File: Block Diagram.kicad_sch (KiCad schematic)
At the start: 0 parts

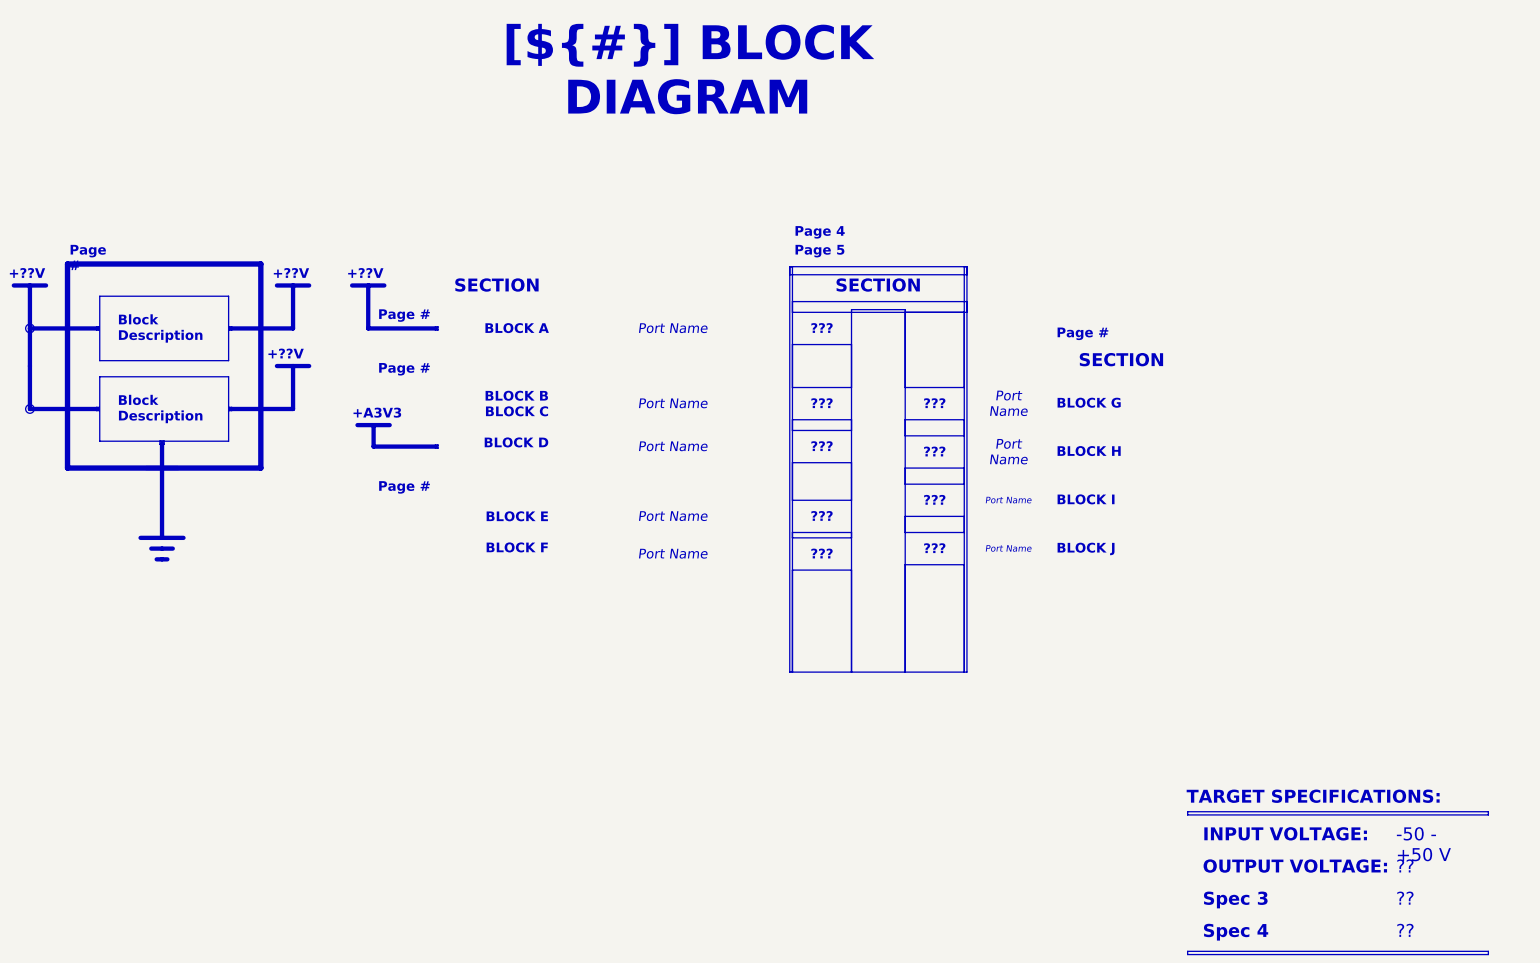
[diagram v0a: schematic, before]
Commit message: fix: template changes
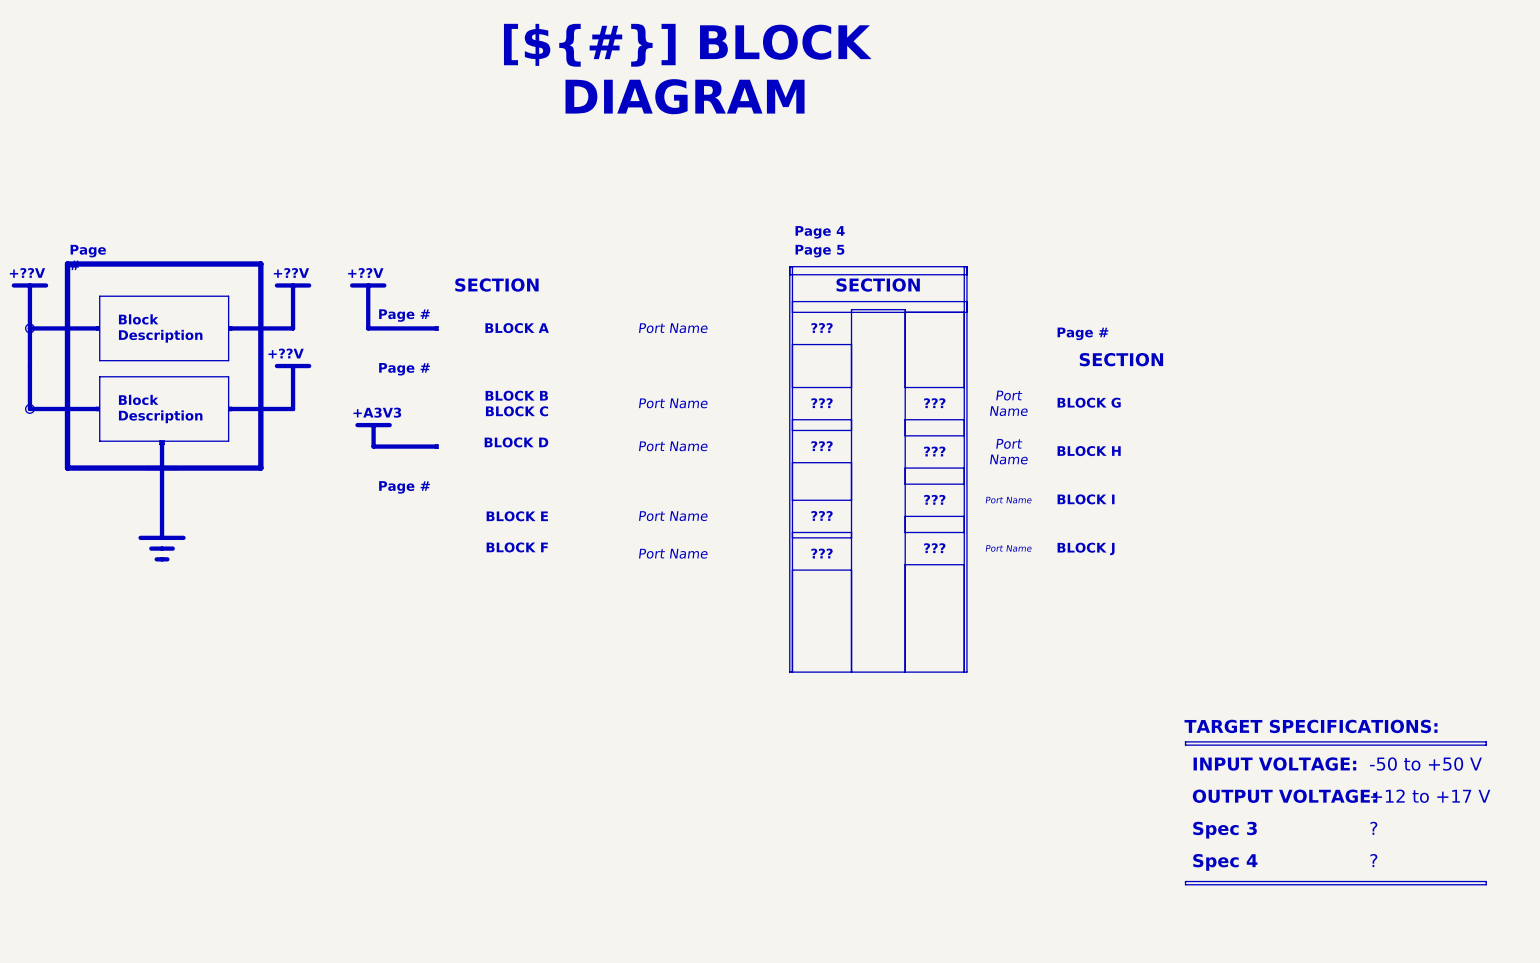
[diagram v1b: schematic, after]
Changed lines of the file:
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@@
 	)
 	(rectangle
-		(start 328.422 234.95)
-		(end 399.542 235.712)
+		(start 327.914 218.44)
+		(end 399.034 219.202)
 		(stroke
 			(width 0)
@@
 	)
 	(rectangle
-		(start 328.422 201.93)
-		(end 399.542 202.692)
+		(start 327.914 185.42)
+		(end 399.034 186.182)
 		(stroke
 			(width 0)
@@
 		)
 	)
+	(text_box "?"
+		(exclude_from_sim no)
+		(at 369.062 201.93 0)
+		(size 38.608 7.62)
+		(margins 2.2859 2.2859 2.2859 2.2859)
+		(stroke
+			(width -0.0001)
+			(type solid)
+		)
+		(fill
+			(type none)
+		)
+		(effects
+			(font
+				(size 3.048 3.048)
+				(color 0 0 0 1)
+			)
+			(justify left top)
+		)
+	)
 	(text_box "SECTION"
 		(exclude_from_sim no)
@@
 	(text_box "Spec 4"
 		(exclude_from_sim no)
-		(at 329.692 226.06 0)
+		(at 327.152 209.55 0)
 		(size 44.45 7.62)
 		(margins 2.2859 2.2859 2.2859 2.2859)
@@
 		(effects
 			(font
-				(face "Times New Roman")
 				(size 3.048 3.048)
 				(thickness 0.4572)
@@
 		)
 	)
-	(text_box "-50 - +50 V"
-		(exclude_from_sim no)
-		(at 375.412 203.2 0)
-		(size 25.908 7.62)
+	(text_box "-50 to +50 V"
+		(exclude_from_sim no)
+		(at 369.062 186.69 0)
+		(size 38.608 7.62)
 		(margins 2.2859 2.2859 2.2859 2.2859)
 		(stroke
@@
 		(effects
 			(font
-				(face "Times New Roman")
+				(size 3.048 3.048)
+				(color 0 0 0 1)
+			)
+			(justify left top)
+		)
+	)
+	(text_box "?"
+		(exclude_from_sim no)
+		(at 369.062 209.55 0)
+		(size 38.608 7.62)
+		(margins 2.2859 2.2859 2.2859 2.2859)
+		(stroke
+			(width -0.0001)
+			(type solid)
+		)
+		(fill
+			(type none)
+		)
+		(effects
+			(font
 				(size 3.048 3.048)
 				(color 0 0 0 1)
@@
 		)
 	)
-	(text_box "??"
-		(exclude_from_sim no)
-		(at 375.412 226.06 0)
-		(size 24.13 7.62)
-		(margins 2.2859 2.2859 2.2859 2.2859)
-		(stroke
-			(width -0.0001)
-			(type default)
-		)
-		(fill
-			(type none)
-		)
-		(effects
-			(font
-				(face "Times New Roman")
+	(text_box "+12 to +17 V"
+		(exclude_from_sim no)
+		(at 369.062 194.31 0)
+		(size 38.608 7.62)
+		(margins 2.2859 2.2859 2.2859 2.2859)
+		(stroke
+			(width -0.0001)
+			(type solid)
+		)
+		(fill
+			(type none)
+		)
+		(effects
+			(font
 				(size 3.048 3.048)
 				(color 0 0 0 1)
@@
 	(text_box "[${#}] ${TITLE}"
 		(exclude_from_sim no)
-		(at 144.78 20.32 0)
-		(size 130.81 12.7)
+		(at 142.24 20.32 0)
+		(size 134.62 12.7)
 		(margins 5.9999 5.9999 5.9999 5.9999)
 		(stroke
@@
 		(effects
 			(font
-				(face "Times New Roman")
 				(size 8 8)
 				(thickness 1.2)
@@
 		)
 	)
-	(text_box "??"
-		(exclude_from_sim no)
-		(at 375.412 210.82 0)
-		(size 24.13 7.62)
-		(margins 2.2859 2.2859 2.2859 2.2859)
-		(stroke
-			(width -0.0001)
-			(type default)
-		)
-		(fill
-			(type none)
-		)
-		(effects
-			(font
-				(face "Times New Roman")
-				(size 3.048 3.048)
-				(color 0 0 0 1)
-			)
-			(justify left top)
-		)
-	)
 	(text_box "INPUT VOLTAGE:"
 		(exclude_from_sim no)
-		(at 329.692 203.2 0)
+		(at 327.152 186.69 0)
 		(size 47.498 7.62)
 		(margins 2.2859 2.2859 2.2859 2.2859)
@@
 		(effects
 			(font
-				(face "Times New Roman")
 				(size 3.048 3.048)
 				(thickness 0.4572)
@@
 	(text_box "TARGET SPECIFICATIONS:"
 		(exclude_from_sim no)
-		(at 325.882 194.31 0)
+		(at 325.374 177.8 0)
 		(size 73.66 7.62)
 		(margins 2.2859 2.2859 2.2859 2.2859)
@@
 		(effects
 			(font
-				(face "Times New Roman")
 				(size 3.048 3.048)
 				(thickness 0.4572)
@@
 	(text_box "Spec 3"
 		(exclude_from_sim no)
-		(at 329.692 218.44 0)
+		(at 327.152 201.93 0)
 		(size 41.91 7.62)
 		(margins 2.2859 2.2859 2.2859 2.2859)
@@
 		(effects
 			(font
-				(face "Times New Roman")
 				(size 3.048 3.048)
 				(thickness 0.4572)
@@
 		)
 	)
-	(text_box "??"
-		(exclude_from_sim no)
-		(at 375.412 218.44 0)
-		(size 24.13 7.62)
-		(margins 2.2859 2.2859 2.2859 2.2859)
-		(stroke
-			(width -0.0001)
-			(type default)
-		)
-		(fill
-			(type none)
-		)
-		(effects
-			(font
-				(face "Times New Roman")
-				(size 3.048 3.048)
-				(color 0 0 0 1)
-			)
-			(justify left top)
-		)
-	)
 	(text_box "OUTPUT VOLTAGE:"
 		(exclude_from_sim no)
-		(at 329.692 210.82 0)
+		(at 327.152 194.31 0)
 		(size 46.228 7.62)
 		(margins 2.2859 2.2859 2.2859 2.2859)
@@
 		(effects
 			(font
-				(face "Times New Roman")
-				(size 3.048 3.048)
-				(thickness 0.4572)
+				(size 3.048 3.048)
+				(thickness 0.4572)
